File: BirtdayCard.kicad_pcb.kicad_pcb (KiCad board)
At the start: 2 copper layers, 32 parts, among them J1 Conn_01x04_Socket, J3 USB_C_Receptacle_USB2.0, Q1 2N7002_C306856, U1 ESP32-C3-WROOM-02-N4(4MB), U2 AMS1117-3.3_C347222

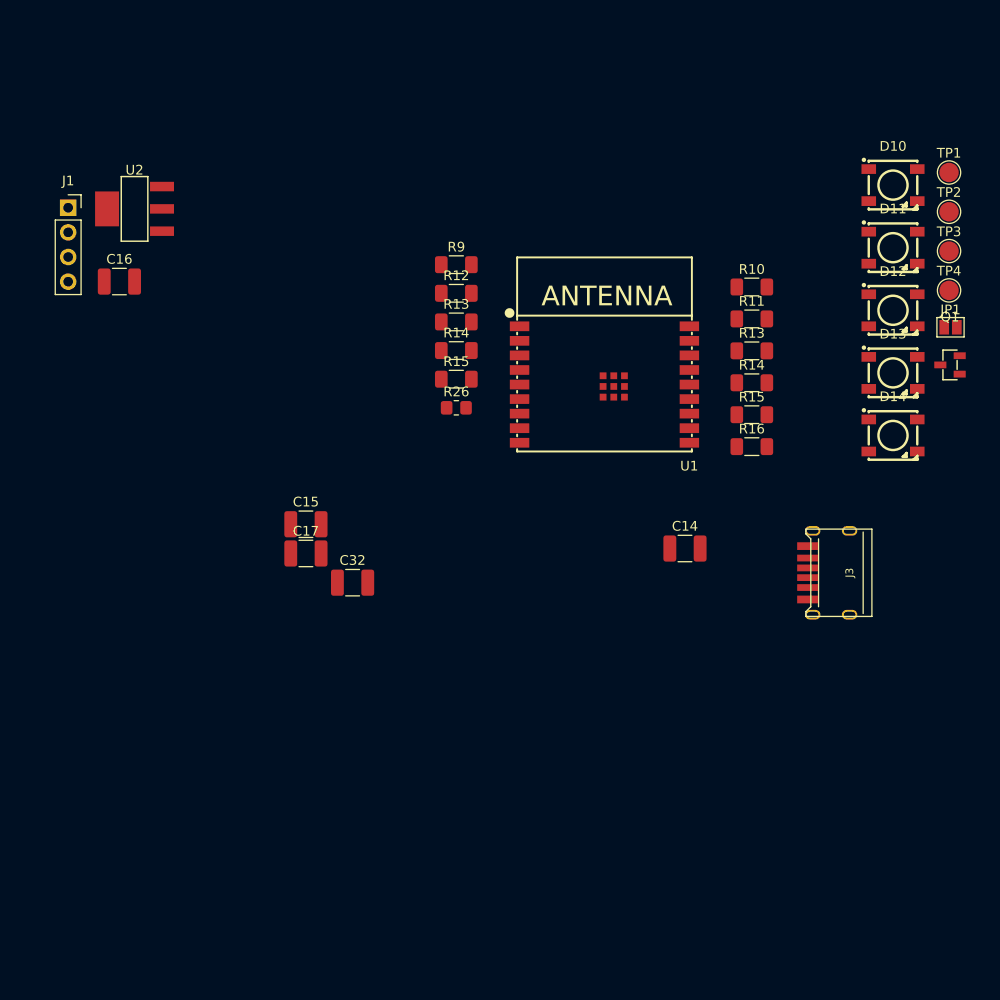
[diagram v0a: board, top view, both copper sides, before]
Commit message: archived 3D models
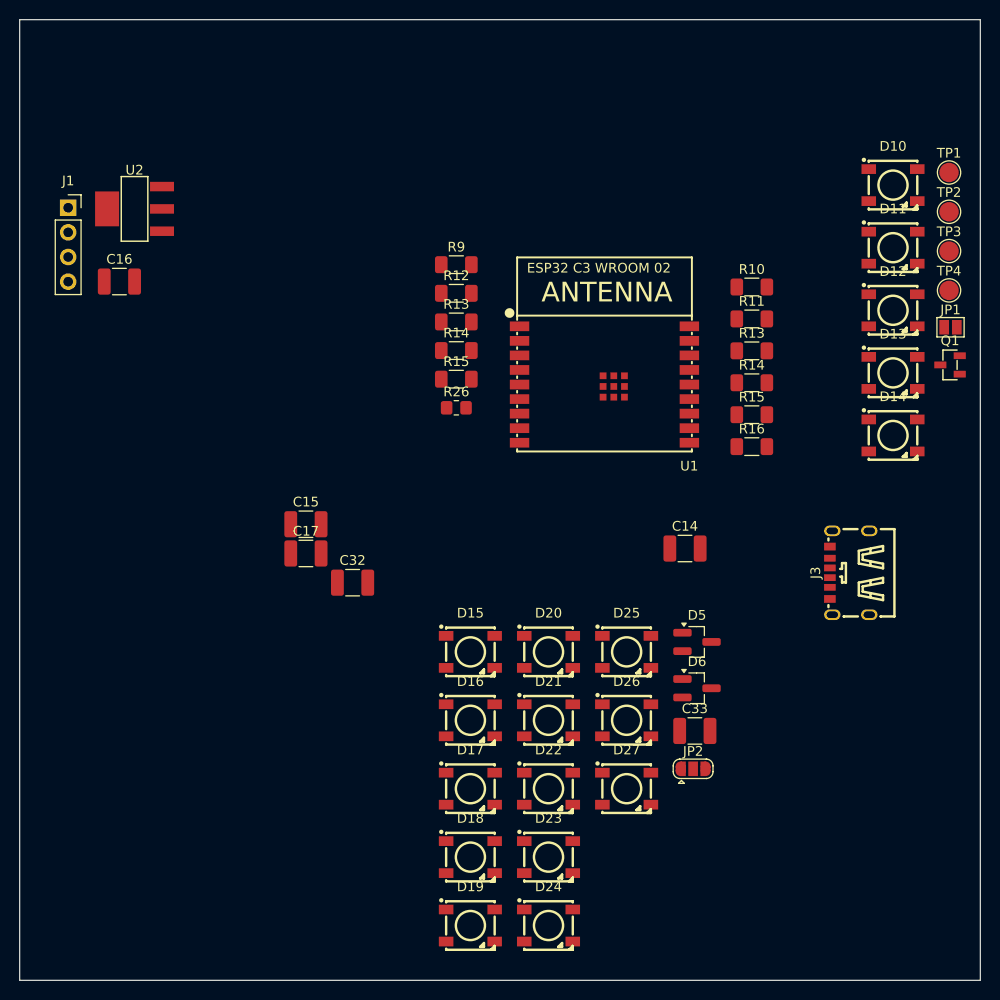
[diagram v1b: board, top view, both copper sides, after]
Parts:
- added C33: 100nF 50V, Capacitor_SMD:C_1210_3225Metric_Pad1.33x2.70mm_HandSolder, F.Cu at (134.6, 105.8)
- added D15: WS2812B, easyeda2kicad:LED-SMD_4P-L5.0-W5.0-BL_TC5050RGB, F.Cu at (111.5, 97.7)
- added D16: WS2812B, easyeda2kicad:LED-SMD_4P-L5.0-W5.0-BL_TC5050RGB, F.Cu at (111.5, 104.7)
- added D17: WS2812B, easyeda2kicad:LED-SMD_4P-L5.0-W5.0-BL_TC5050RGB, F.Cu at (111.5, 111.8)
- added D18: WS2812B, easyeda2kicad:LED-SMD_4P-L5.0-W5.0-BL_TC5050RGB, F.Cu at (111.5, 118.8)
- added D19: WS2812B, easyeda2kicad:LED-SMD_4P-L5.0-W5.0-BL_TC5050RGB, F.Cu at (111.5, 125.8)
- added D20: WS2812B, easyeda2kicad:LED-SMD_4P-L5.0-W5.0-BL_TC5050RGB, F.Cu at (119.5, 97.7)
- added D21: WS2812B, easyeda2kicad:LED-SMD_4P-L5.0-W5.0-BL_TC5050RGB, F.Cu at (119.5, 104.7)
- added D22: WS2812B, easyeda2kicad:LED-SMD_4P-L5.0-W5.0-BL_TC5050RGB, F.Cu at (119.5, 111.8)
- added D23: WS2812B, easyeda2kicad:LED-SMD_4P-L5.0-W5.0-BL_TC5050RGB, F.Cu at (119.5, 118.8)
- added D24: WS2812B, easyeda2kicad:LED-SMD_4P-L5.0-W5.0-BL_TC5050RGB, F.Cu at (119.5, 125.8)
- added D25: WS2812B, easyeda2kicad:LED-SMD_4P-L5.0-W5.0-BL_TC5050RGB, F.Cu at (127.5, 97.7)
- added D26: WS2812B, easyeda2kicad:LED-SMD_4P-L5.0-W5.0-BL_TC5050RGB, F.Cu at (127.5, 104.7)
- added D27: WS2812B, easyeda2kicad:LED-SMD_4P-L5.0-W5.0-BL_TC5050RGB, F.Cu at (127.5, 111.8)
- added D5: 7A 150W, Package_TO_SOT_SMD:SOT-23_Handsoldering, F.Cu at (134.8, 96.6)
- added D6: 7A 150W, Package_TO_SOT_SMD:SOT-23_Handsoldering, F.Cu at (134.8, 101.4)
- added JP2: SolderJumper_3_Open, Jumper:SolderJumper-3_P1.3mm_Open_RoundedPad1.0x1.5mm, F.Cu at (134.4, 109.7)
- J3: footprint USB-C-Power-tester:TYPE-C-31-M-17_handsolder -> easyeda2kicad:TYPE-C-SMD_TYPE-C-6P_5
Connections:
- D14 pad 2: unconnected-(D14-DOUT-Pad2) -> Net-(D14-DOUT)
- R14 pad 1: +3V3 -> GPIO8 (x2)
- R14 pad 2: GPIO8 -> Net-(JP2-C) (x2)
- U1 pad 10: GPIO10 -> BUZZ
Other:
- board outline added: 99 x 99 mm
